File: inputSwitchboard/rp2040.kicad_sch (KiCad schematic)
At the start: 31 parts, among them J10 BOOTSEL, J11 RESET, J12 DEBUG, U10 W25Q128JVS, U2 RP2040, U9 TXS0108EPW, Y1 ABM8-272-T3

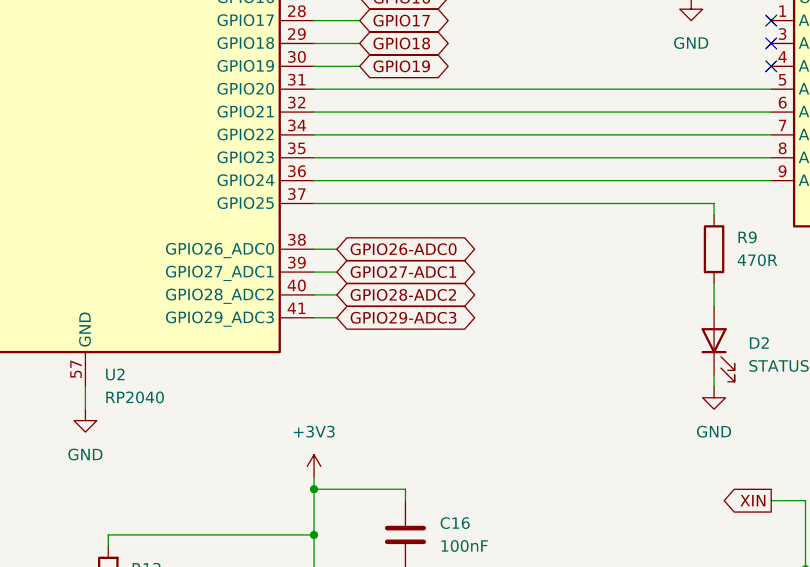
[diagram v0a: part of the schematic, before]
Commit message: finished routing
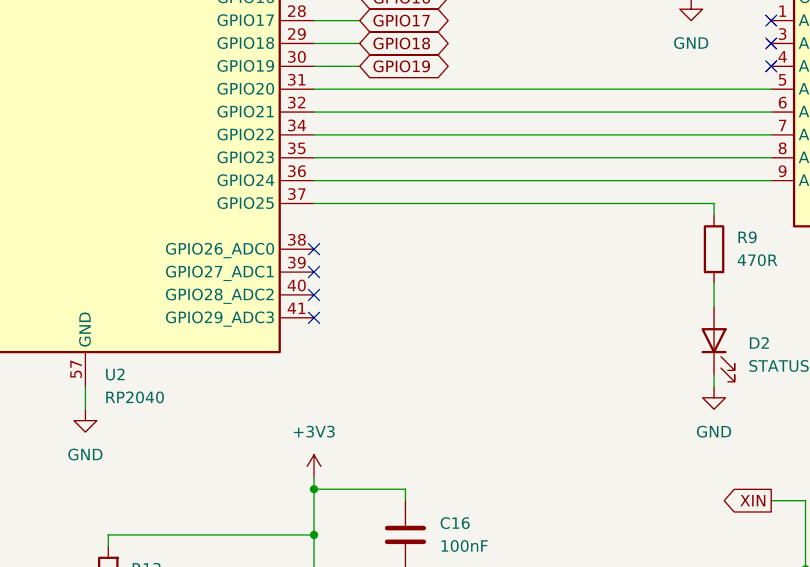
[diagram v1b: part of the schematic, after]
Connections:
- net GPIO26-ADC0: no longer names the net of U2.38 (GPIO26_ADC0)
- net GPIO27-ADC1: no longer names the net of U2.39 (GPIO27_ADC1)
- net GPIO28-ADC2: no longer names the net of U2.40 (GPIO28_ADC2)
- net GPIO29-ADC3: no longer names the net of U2.41 (GPIO29_ADC3)
- no-connect marks 8 -> 12
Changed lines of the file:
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@@
+	)
+	(no_connect
+		(at 109.22 118.11)
 	)
 	(no_connect
@@
 	)
 	(no_connect
+		(at 109.22 113.03)
+	)
+	(no_connect
 		(at 160.02 87.63)
 	)
@@
 	)
 	(no_connect
+		(at 109.22 115.57)
+	)
+	(no_connect
 		(at 180.34 87.63)
 	)
+	(no_connect
+		(at 109.22 110.49)
+	)
 	(wire
 		(pts
@@
 	(wire
 		(pts
-			(xy 111.76 113.03) (xy 109.22 113.03)
-		)
-		(stroke
-			(width 0)
-			(type default)
-		)
-	)
-	(wire
-		(pts
 			(xy 109.22 85.09) (xy 114.3 85.09)
 		)
@@
 	(wire
 		(pts
-			(xy 111.76 110.49) (xy 109.22 110.49)
-		)
-		(stroke
-			(width 0)
-			(type default)
-		)
-	)
-	(wire
-		(pts
 			(xy 109.22 137.16) (xy 109.22 142.24)
 		)
@@
 	(wire
 		(pts
-			(xy 111.76 115.57) (xy 109.22 115.57)
-		)
-		(stroke
-			(width 0)
-			(type default)
-		)
-	)
-	(wire
-		(pts
 			(xy 163.83 138.43) (xy 163.83 146.05)
 		)
@@
 		(pts
 			(xy 195.58 156.21) (xy 195.58 157.48)
-		)
-		(stroke
-			(width 0)
-			(type default)
-		)
-	)
-	(wire
-		(pts
-			(xy 111.76 118.11) (xy 109.22 118.11)
 		)
 		(stroke
@@
 		)
 	)
-	(global_label "GPIO29-ADC3"
-		(shape bidirectional)
-		(at 111.76 118.11 0)
-		(fields_autoplaced yes)
-		(effects
-			(font
-				(size 1.27 1.27)
-			)
-			(justify left)
-		)
-		(property "Intersheetrefs" "${INTERSHEET_REFS}"
-			(at 129.1613 118.11 0)
-			(effects
-				(font
-					(size 1.27 1.27)
-				)
-				(justify left)
-				(hide yes)
-			)
-		)
-	)
-	(global_label "GPIO26-ADC0"
-		(shape bidirectional)
-		(at 111.76 110.49 0)
-		(fields_autoplaced yes)
-		(effects
-			(font
-				(size 1.27 1.27)
-			)
-			(justify left)
-		)
-		(property "Intersheetrefs" "${INTERSHEET_REFS}"
-			(at 129.1613 110.49 0)
-			(effects
-				(font
-					(size 1.27 1.27)
-				)
-				(justify left)
-				(hide yes)
-			)
-		)
-	)
 	(global_label "GPIO14"
 		(shape bidirectional)
@@
 		)
 	)
-	(global_label "GPIO27-ADC1"
-		(shape bidirectional)
-		(at 111.76 113.03 0)
-		(fields_autoplaced yes)
-		(effects
-			(font
-				(size 1.27 1.27)
-			)
-			(justify left)
-		)
-		(property "Intersheetrefs" "${INTERSHEET_REFS}"
-			(at 129.1613 113.03 0)
-			(effects
-				(font
-					(size 1.27 1.27)
-				)
-				(justify left)
-				(hide yes)
-			)
-		)
-	)
 	(global_label "NAND-SCLK"
 		(shape output)
@@
 				(hide yes)
 			)
-		)
-	)
-	(global_label "GPIO28-ADC2"
-		(shape bidirectional)
-		(at 111.76 115.57 0)
-		(fields_autoplaced yes)
-		(effects
-			(font
-				(size 1.27 1.27)
-			)
-			(justify left)
-		)
-		(property "Intersheetrefs" "${INTERSHEET_REFS}"
-			(at 129.1613 115.57 0)
-			(effects
-				(font
-					(size 1.27 1.27)
-				)
-				(justify left)
-				(hide yes)
-			)

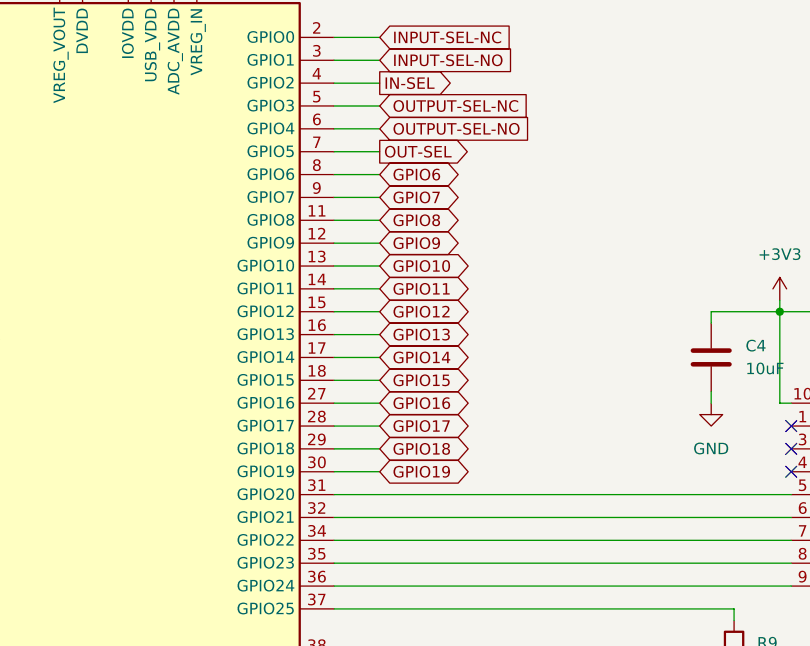
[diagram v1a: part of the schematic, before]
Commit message: fixed more stuff and polished routing
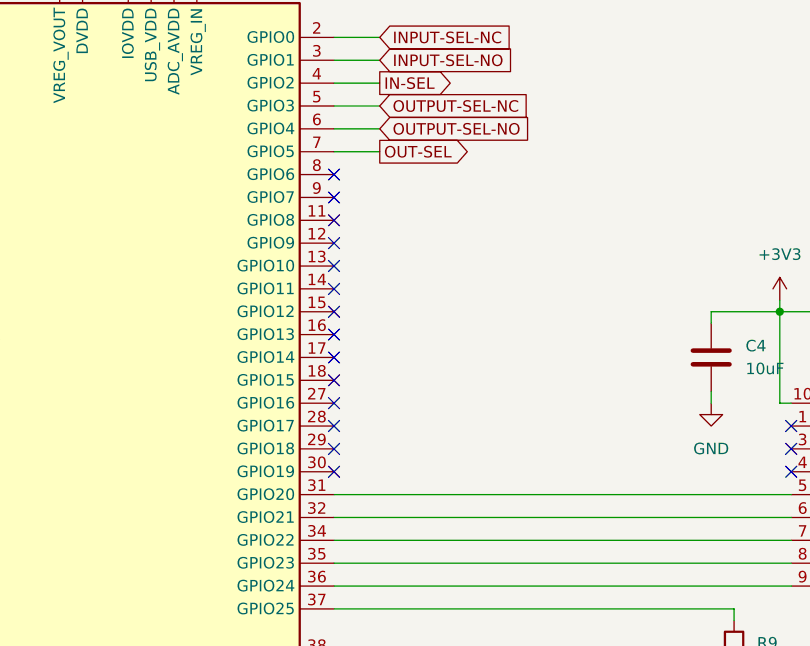
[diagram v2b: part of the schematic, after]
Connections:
- net GPIO10: no longer names the net of U2.13 (GPIO10)
- net GPIO11: no longer names the net of U2.14 (GPIO11)
- net GPIO12: no longer names the net of U2.15 (GPIO12)
- net GPIO13: no longer names the net of U2.16 (GPIO13)
- net GPIO14: no longer names the net of U2.17 (GPIO14)
- net GPIO15: no longer names the net of U2.18 (GPIO15)
- net GPIO16: no longer names the net of U2.27 (GPIO16)
- net GPIO17: no longer names the net of U2.28 (GPIO17)
- net GPIO18: no longer names the net of U2.29 (GPIO18)
- net GPIO19: no longer names the net of U2.30 (GPIO19)
- net GPIO6: no longer names the net of U2.8 (GPIO6)
- net GPIO7: no longer names the net of U2.9 (GPIO7)
- net GPIO8: no longer names the net of U2.11 (GPIO8)
- net GPIO9: no longer names the net of U2.12 (GPIO9)
- no-connect marks 12 -> 26

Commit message: done!
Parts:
- D2: footprint LED_SMD:LED_0201_0603Metric -> LED_SMD:LED_0603_1608Metric
- Y1: footprint imports:XTAL_ABM8-272-T3 -> ABM8-272-T3:XTAL_ABM8-272-T3
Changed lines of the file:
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@@
 			)
 		)
-		(property "Footprint" "LED_SMD:LED_0201_0603Metric"
+		(property "Footprint" "LED_SMD:LED_0603_1608Metric"
 			(at 153.67 120.65 0)
 			(effects
@@
 			)
 		)
-		(property "Footprint" "imports:XTAL_ABM8-272-T3"
+		(property "Footprint" "ABM8-272-T3:XTAL_ABM8-272-T3"
 			(at 179.07 146.05 0)
 			(effects
